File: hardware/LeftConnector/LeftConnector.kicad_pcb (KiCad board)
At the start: 2 copper layers, 22.8 x 14.8 mm, 4 parts, among them J1 Conn_01x10, J2 Conn_01x10

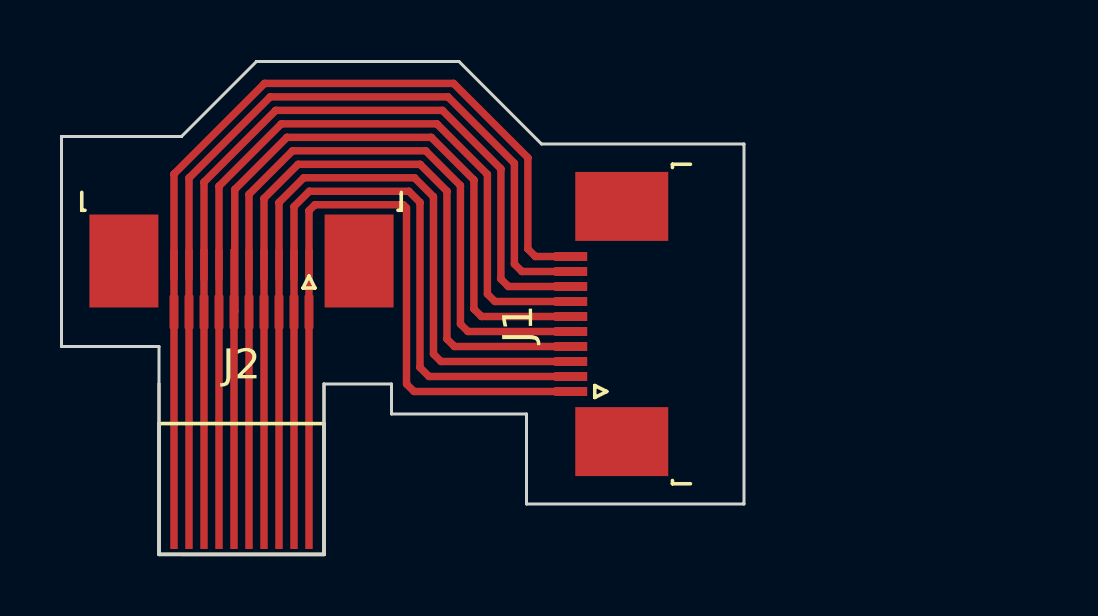
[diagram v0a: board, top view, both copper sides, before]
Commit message: Left connector initial FPC
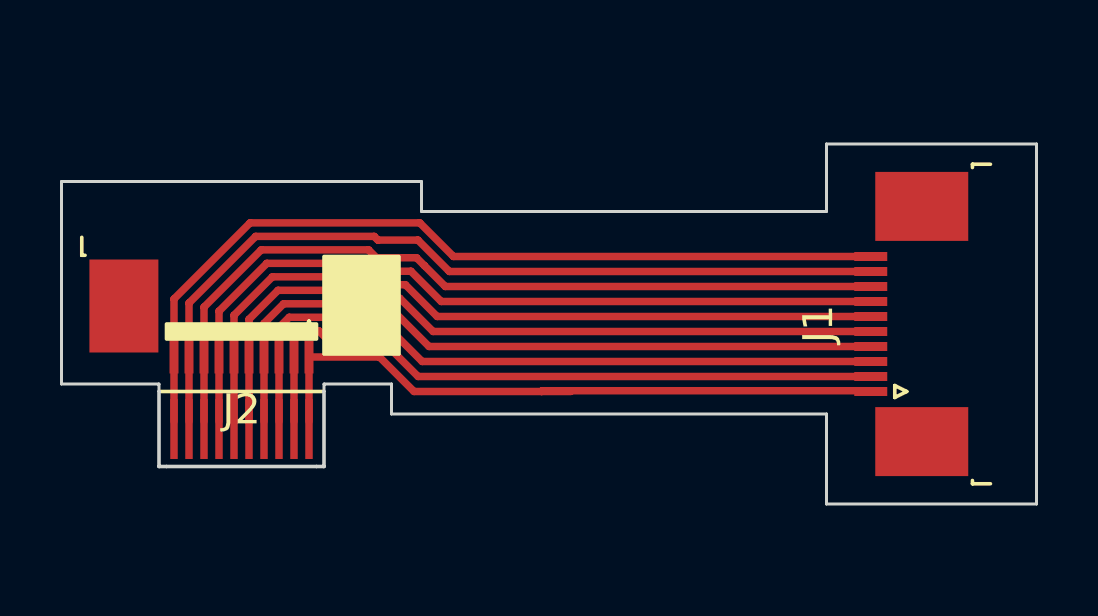
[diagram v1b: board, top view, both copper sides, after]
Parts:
- removed G***: LOGO, consolizer:QR
- C1: footprint consolizer:flex_long_10 -> consolizer:flex_short_10
- moved J1 10.00 mm to (131.3, 82.8)
- moved J2 1.50 mm to (109.0, 82.5)
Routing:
- net /C1P10: track 22.1 -> 29.2 mm
- net /C1P9: track 21.6 -> 28.4 mm
- net /C1P8: track 21.0 -> 27.7 mm
- net /C1P7: track 20.5 -> 26.9 mm
- net /C1P5: track 19.3 -> 25.5 mm
- net /C1P4: track 18.8 -> 24.7 mm
- net /C1P3: track 18.2 -> 24.0 mm
- net /C1P1: track 17.1 -> 22.7 mm
- net /C1P2: track 17.6 -> 23.2 mm
- net /C1P6: track 21.0 -> 26.2 mm
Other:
- board size 22.8 x 14.8 mm -> 32.5 x 12 mm
